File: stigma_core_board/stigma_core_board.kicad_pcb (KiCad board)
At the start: 4 copper layers, 40 x 40 mm, 93 parts, among them J1 TC2050, J5 USB_C_Receptacle_USB2.0, SW1 KMR721NGLFS, SW2 KMR721NGLFS, U1 STM32H743VITx, U10 H3LIS331DL, U11 MS5607/MS5611, U12 LIS3MDL, U13 BMP580, U2 TPD4E1U06, U3 LPS22, U4 ICM-42670-P, U5 AZ1117I-3.3, U6 ICM-42688-P, U7 TPD4E1U06, U8 W25Q128JVP, U9 LSM6DSR, Y1 25MHz, Y2 32.768kHz

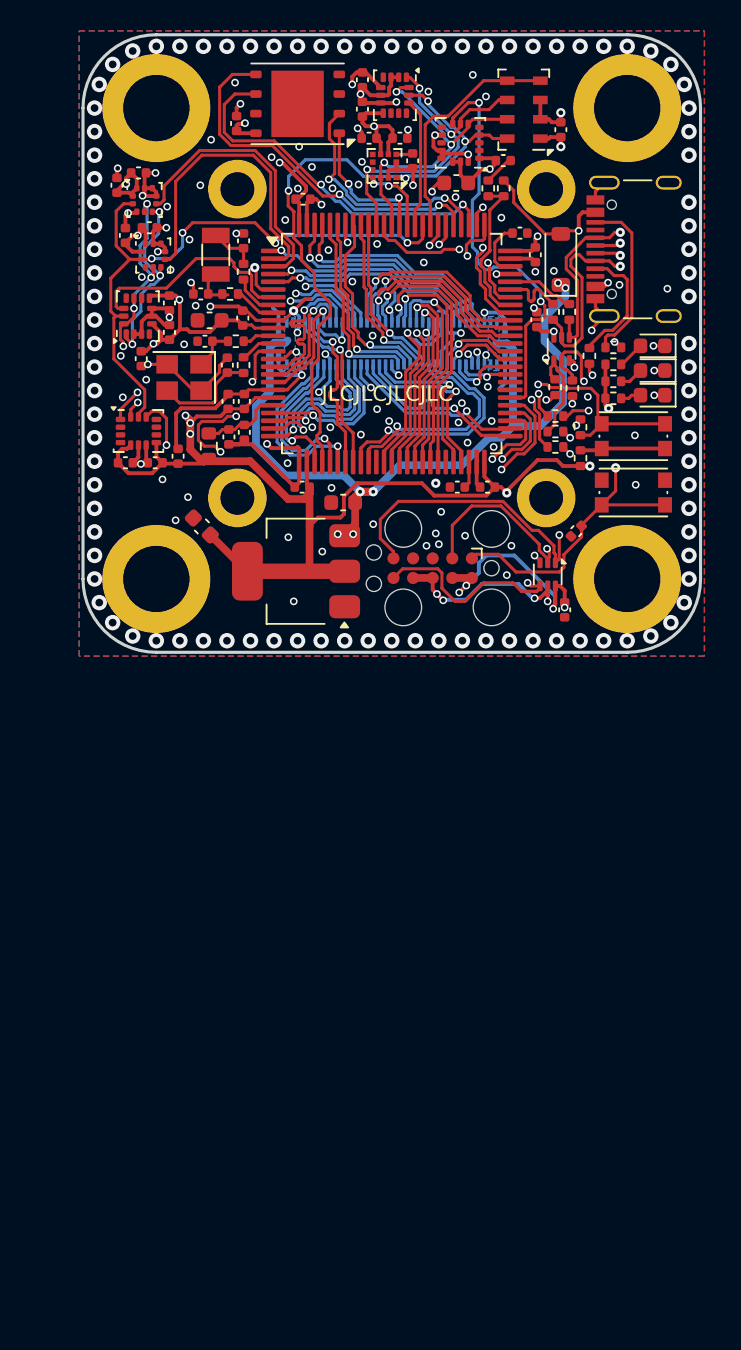
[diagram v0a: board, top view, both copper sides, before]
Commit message: uploaded files to share current not working parts
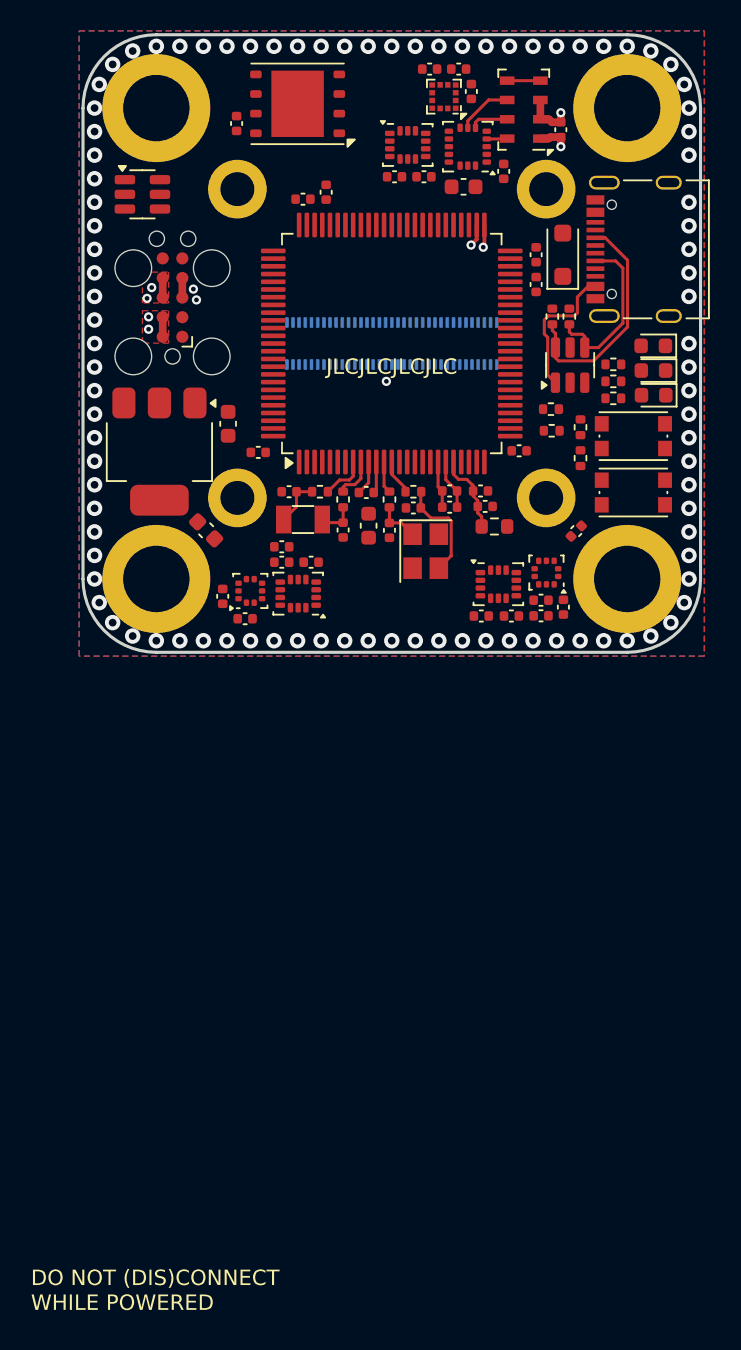
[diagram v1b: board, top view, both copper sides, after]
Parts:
- removed C39, C40: 100n, Capacitor_SMD:C_0402_1005Metric
- removed J3: ~, stigma:DF40GB-70DP-0.4V-plug
- removed R14: 4k7, Resistor_SMD:R_0402_1005Metric
- removed R15: 10k, Resistor_SMD:R_0402_1005Metric
- removed R16, R17, R18, R19, R20: 22, Resistor_SMD:R_0402_1005Metric
- removed U7: TPD4E1U06, Package_TO_SOT_SMD:SOT-563
- added REF**: DF40GB-70DP-0.4V, stigma:DF40GB-70DP-0.4V, B.Cu at (117.5, 115.2)
- added U2: TPD4E1U06, Package_TO_SOT_SMD:SOT-23-6, F.Cu at (99.1, 105.6)
- D1: value red -> LED_Small
- D2: value yellow -> LED_Small
- D3: value green -> LED_Small
- D4: footprint Diode_SMD:D_SOD-123 -> Diode_SMD:D_SOD-123F
- R7, R8, R9: value 1k -> 680
- U13: value BMP580 -> BMP580/BMP388/LPS22
- U2: footprint Package_TO_SOT_SMD:SOT-563 -> Package_TO_SOT_SMD:SOT-23-6
- U3: value LPS22 -> BMP580/BMP388/LPS22
- U4: value ICM-42670-P -> IIM-42652 (or other LGA-14 IMU)
- U6: value ICM-42688-P -> ICM-42688 (or other LGA-14 IMU)
- moved C30 39.3 mm to (126.4, 132.3), turned to 90 degrees
- moved C29 38.4 mm to (124.9, 131.9), turned to 0 degrees
- moved U3 35.5 mm to (125.3, 130.1), turned to 180 degrees
- moved C35 26.0 mm to (105.8, 133.1), turned to 180 degrees
- moved C37 25.7 mm to (124.9, 132.9), turned to 180 degrees
- moved U6 25.3 mm to (122.2, 130.8)
- moved C31 25.1 mm to (123.0, 132.9)
- moved C32 25.1 mm to (121.0, 132.9)
- moved C36 24.3 mm to (104.3, 131.6), turned to -90 degrees
- moved J1 24.3 mm to (101.0, 112.3), turned to 90 degrees
- moved U13 22.6 mm to (106.1, 131.3), turned to 90 degrees
- moved U4 20.8 mm to (109.2, 131.4), turned to 180 degrees
- moved Y1 19.3 mm to (117.5, 128.7), turned to -90 degrees
- moved FB1 19.2 mm to (121.9, 127.1), turned to 180 degrees
- moved C34 18.3 mm to (108.1, 129.4), turned to 0 degrees
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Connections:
- net /VCAP1 renamed Net-(C9-Pad1)
- net /VCAP2 renamed Net-(C10-Pad1)
- C19 pad 2: +3.3V -> +3V3
- C21 pad 2: +3.3V -> +3V3
- C22 pad 2: +3.3V -> +3V3
- C23 pad 2: +3.3V -> +3V3
- C24 pad 2: +3.3V -> +3V3
- C25 pad 2: +3.3V -> +3V3
- C26 pad 2: +3.3V -> +3V3
- C27 pad 2: +3.3V -> +3V3
- C29 pad 2: +3.3V -> +3V3
- C30 pad 2: +3.3V -> +3V3
- C31 pad 2: +3.3V -> +3V3
- C32 pad 2: +3.3V -> +3V3
- C33 pad 2: +3.3V -> +3V3
- C34 pad 2: +3.3V -> +3V3
- C35 pad 2: +3.3V -> +3V3
- C36 pad 2: +3.3V -> +3V3
- C37 pad 2: +3.3V -> +3V3
- C38 pad 2: +3.3V -> +3V3
- D4 pad 2: /VBUS -> Net-(D4-A)
- J1 pad 2: /J1-SWDIO -> SWDIO
- J1 pad 5: /J1-SWO -> SWO
- J1 pad 6: Net-(J1-Pin_6) -> SWCLK
- J5 pad A4: /VBUS -> Net-(D4-A)
- J5 pad A9: /VBUS -> Net-(D4-A)
- J5 pad B4: /VBUS -> Net-(D4-A)
- J5 pad B9: /VBUS -> Net-(D4-A)
- R6 pad 2: +3.3V -> +3V3
- U1 pad 1: PE2 -> SPI4_SCK
- U1 pad 14: Net-(U1-NRST) -> NRST
- U1 pad 15: PC0 -> unconnected-(U1-PC0-Pad15)
- U1 pad 16: PC1_ETH_MDC -> ETH_MDC
- U1 pad 17: PC2_C -> SPI2_MISO
- U1 pad 18: PC3_C -> SPI2_MOSI
- U1 pad 2: SPI2_CS_BARO3 -> unconnected-(U1-PE3-Pad2)
- U1 pad 22: PA0 -> unconnected-(U1-PA0-Pad22)
- U1 pad 23: PA1_ETH_REF_CLK -> ETH_REF_CLK
- U1 pad 24: PA2_ETH_MDIO -> ETH_MDIO
- U1 pad 25: PA3 -> unconnected-(U1-PA3-Pad25)
- U1 pad 28: PA4 -> unconnected-(U1-PA4-Pad28)
- U1 pad 3: SPI2_CS_BARO2 -> unconnected-(U1-PE4-Pad3)
- U1 pad 30: PA6 -> SPI1_MISO
- U1 pad 31: PA7_ETH_CRS_DV -> ETH_CRS_DV
- U1 pad 32: ETH_RXD- -> ETH_RXD0
- U1 pad 33: ETH_RXD+ -> ETH_RXD1
- U1 pad 34: PB0 -> unconnected-(U1-PB0-Pad34)
- U1 pad 35: PB1 -> unconnected-(U1-PB1-Pad35)
- U1 pad 37: PE7 -> unconnected-(U1-PE7-Pad37)
- U1 pad 38: PE8 -> unconnected-(U1-PE8-Pad38)
- U1 pad 39: PE9 -> unconnected-(U1-PE9-Pad39)
- U1 pad 4: PE5 -> SPI4_MISO
- U1 pad 40: PE10 -> unconnected-(U1-PE10-Pad40)
- U1 pad 41: PE11 -> unconnected-(U1-PE11-Pad41)
- U1 pad 42: PE12 -> unconnected-(U1-PE12-Pad42)
- U1 pad 43: PE13 -> unconnected-(U1-PE13-Pad43)
- U1 pad 44: PE14 -> unconnected-(U1-PE14-Pad44)
- U1 pad 46: PB10 -> unconnected-(U1-PB10-Pad46)
- U1 pad 47: PB11_ETH_TX_EN -> ETH_TX_EN
- U1 pad 5: PE6 -> SPI4_MOSI
- U1 pad 51: ETH_TXD- -> ETH_TXD0
- U1 pad 52: ETH_TXD+ -> ETH_TXD1
- U1 pad 53: SPI2_MISO -> USB_D-
- U1 pad 54: SPI2_MOSI -> USB_D+
- U1 pad 55: SPI2_CS_IMU2 -> unconnected-(U1-PD8-Pad55)
- U1 pad 56: SPI1_CS_HIGHG -> unconnected-(U1-PD9-Pad56)
- U1 pad 59: PD12 -> unconnected-(U1-PD12-Pad59)
- U1 pad 60: PD13 -> unconnected-(U1-PD13-Pad60)
- U1 pad 61: PD14 -> unconnected-(U1-PD14-Pad61)
- U1 pad 62: PD15 -> unconnected-(U1-PD15-Pad62)
- U1 pad 63: PC6 -> unconnected-(U1-PC6-Pad63)
- U1 pad 64: PC7 -> unconnected-(U1-PC7-Pad64)
- U1 pad 65: PC8 -> unconnected-(U1-PC8-Pad65)
- U1 pad 66: PC9 -> unconnected-(U1-PC9-Pad66)
- U1 pad 67: LED_RED -> unconnected-(U1-PA8-Pad67)
- U1 pad 69: LED_YELLOW -> unconnected-(U1-PA10-Pad69)
- U1 pad 7: SPI2_CS_IMU3 -> unconnected-(U1-PC13-Pad7)
- U1 pad 70: USB_D- -> CAN1_RX
- U1 pad 71: USB_D+ -> CAN1_TX
- U1 pad 77: LED_GREEN -> unconnected-(U1-PA15-Pad77)
- U1 pad 81: PD0 -> unconnected-(U1-PD0-Pad81)
- U1 pad 82: PD1 -> unconnected-(U1-PD1-Pad82)
- U1 pad 83: SPI1_CS_BARO1 -> unconnected-(U1-PD2-Pad83)
- U1 pad 85: SPI1_CS_IMU1 -> unconnected-(U1-PD4-Pad85)
- U1 pad 86: SPI1_CS_MAG -> unconnected-(U1-PD5-Pad86)
- U1 pad 87: SPI3_CS_FLASH -> unconnected-(U1-PD6-Pad87)
- U1 pad 90: SPI1_MISO -> unconnected-(U1-PB4-Pad90)
- U1 pad 91: PB5 -> CAN2_RX
- U1 pad 92: PB6 -> CAN2_TX
- U1 pad 93: PB7 -> unconnected-(U1-PB7-Pad93)
- U1 pad 94: Net-(U1-BOOT0) -> BOOT0
- U1 pad 95: PB8 -> unconnected-(U1-PB8-Pad95)
- U1 pad 96: PB9 -> unconnected-(U1-PB9-Pad96)
- U1 pad 97: PE0 -> unconnected-(U1-PE0-Pad97)
- U1 pad 98: PE1 -> unconnected-(U1-PE1-Pad98)
- U10 pad 1: +3.3V -> +3V3
- U10 pad 14: +3.3V -> +3V3
- U10 pad 15: +3.3V -> +3V3
- U10 pad 4: SPI1_SCK -> SPI1_SCL
- U10 pad 8: SPI1_CS_HIGHG -> SPI1_CS_ACC
- U11 pad 1: +3.3V -> +3V3
- U11 pad 8: SPI1_SCK -> SPI1_SCL
- U12 pad 1: SPI1_SCK -> SPI1_SCL
- U12 pad 5: +3.3V -> +3V3
- U12 pad 6: +3.3V -> +3V3
- U13 pad 1: +3.3V -> +3V3
- U13 pad 10: +3.3V -> +3V3
- U13 pad 6: SPI2_CS_BARO3 -> SPI1_CS_BARO3
- U2 pad 1: BOOT -> Net-(D4-A)
- U2 pad 2: NRST -> GND
- U2 pad 3: GND -> unconnected-(U2-IO2-Pad3)
- U2 pad 4: /D0+ -> /D0-
- U2 pad 5: /D0- -> unconnected-(U2-VP-Pad5)
- U2 pad 6: /VBUS -> /D0+
- U3 pad 1: +3.3V -> +3V3
- U3 pad 10: +3.3V -> +3V3
- U3 pad 6: SPI2_CS_BARO2 -> SPI1_CS_BARO2
- U4 pad 12: SPI2_CS_IMU3 -> SPI1_CS_IMU3
- U4 pad 5: +3.3V -> +3V3
- U4 pad 8: +3.3V -> +3V3
- U5 pad 2: +3.3V -> +3V3
- U6 pad 12: SPI2_CS_IMU2 -> SPI1_CS_IMU2
- U6 pad 5: +3.3V -> +3V3
- U6 pad 8: +3.3V -> +3V3
- U9 pad 13: SPI1_SCK -> SPI1_SCL
- U9 pad 5: +3.3V -> +3V3
- U9 pad 8: +3.3V -> +3V3
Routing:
- net +3.3V: track 231.6 -> 6.54 mm, vias 22 -> 2
- net GND: track 123.4 -> 9.82 mm, vias 203 -> 98
- net +5V: track 85.8 -> 1.27 mm, vias 10 -> 2
- net SPI2_MOSI: track 50.7 -> 0.00 mm, vias 6 -> 0
- net SPI2_MISO: track 50.1 -> 0.00 mm, vias 5 -> 0
- net Net-(U1-NRST): track 44.1 -> 0.00 mm, vias 4 -> 0
- net SPI3_MOSI: track 43.9 -> 0.00 mm, vias 3 -> 0
- net SPI1_SCK: track 42.9 -> 0.00 mm, vias 4 -> 0
- net SPI2_SCK: track 39.6 -> 0.00 mm, vias 4 -> 0
- net SPI3_SCK: track 39.5 -> 0.00 mm, vias 3 -> 0
- net SPI2_CS_IMU2: track 34.9 -> 0.00 mm, vias 2 -> 0
- net SPI3_MISO: track 32.8 -> 0.00 mm, vias 3 -> 0
- net NRST: track 31.8 -> 0.00 mm, vias 2 -> 0
- net LED_GREEN: track 28.1 -> 0.00 mm, vias 2 -> 0
- net /J1-SWDIO: track 27.7 -> 0.00 mm, vias 2 -> 0
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- added copper zone on F.Cu, net +3.3V
- added copper zone on F.Cu, net +5V
- removed copper zone on B.Cu, net +5V
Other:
- board text added: "DO NOT (DIS)CONNECT WHILE POWERED"
- board text added: "S/N"
- board text added: "stigma"
